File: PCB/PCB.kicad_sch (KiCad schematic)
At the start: 38 parts, among them J1 USB_B_Mini, J2 Conn_02x03_Odd_Even, J3 OLED, J4 AudioJack3, Q1 MMBF170, Q2 MMBF170, SW1 SW_Push, SW2 SW_Push, SW3 12CE3xxxxxxTx, SW4 SW_SPST, U1 ATtiny261A-M, U2 MCP73832-2-OT

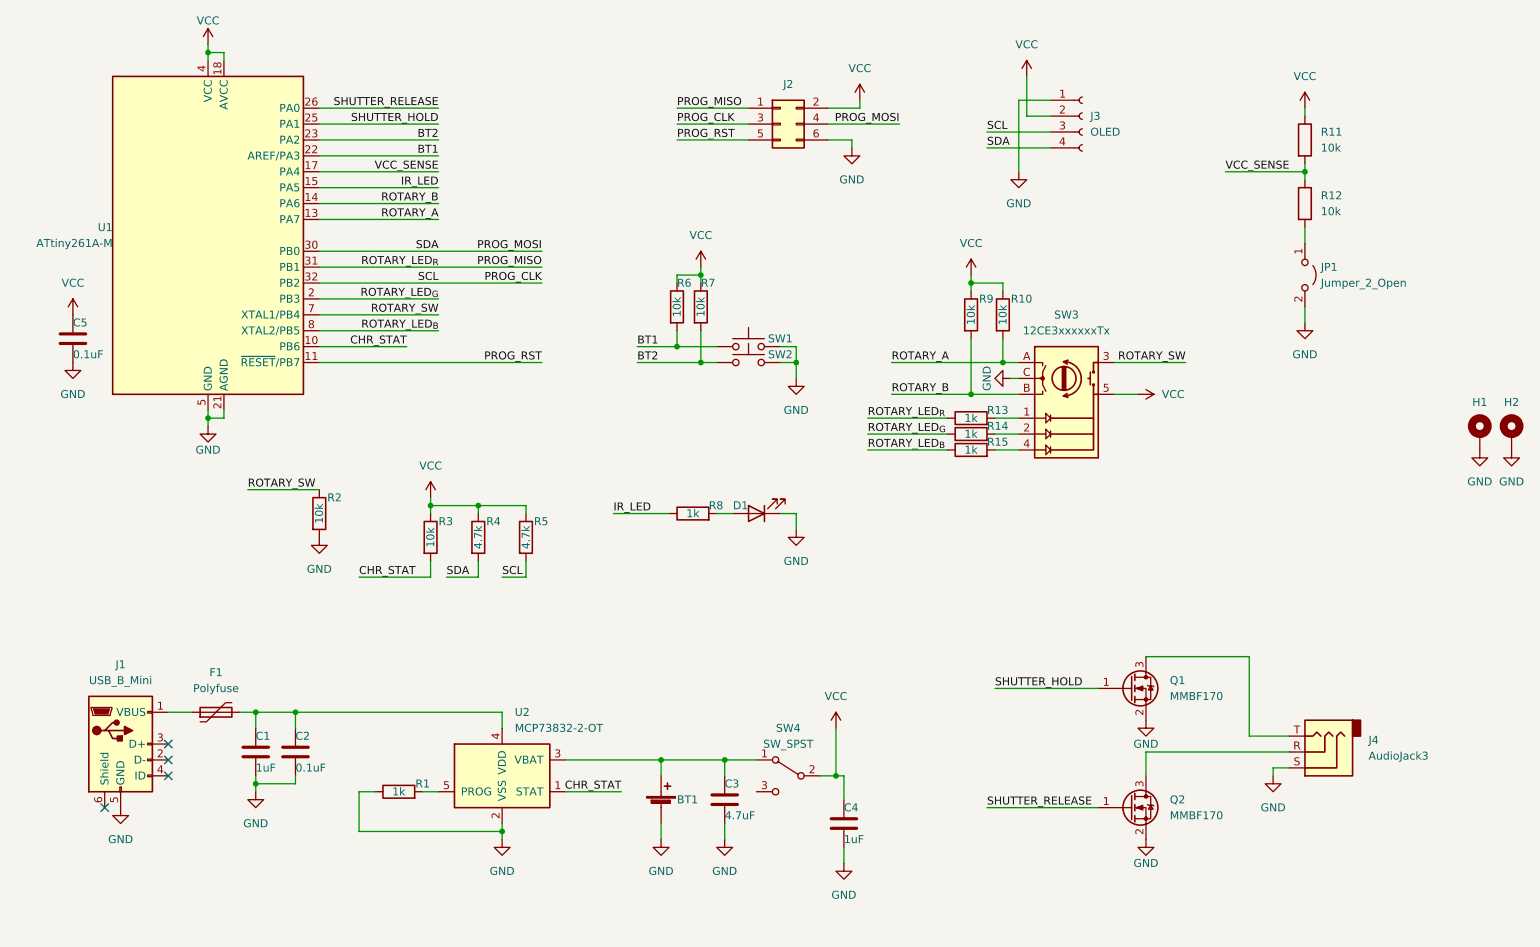
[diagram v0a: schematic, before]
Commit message: Updated schematic
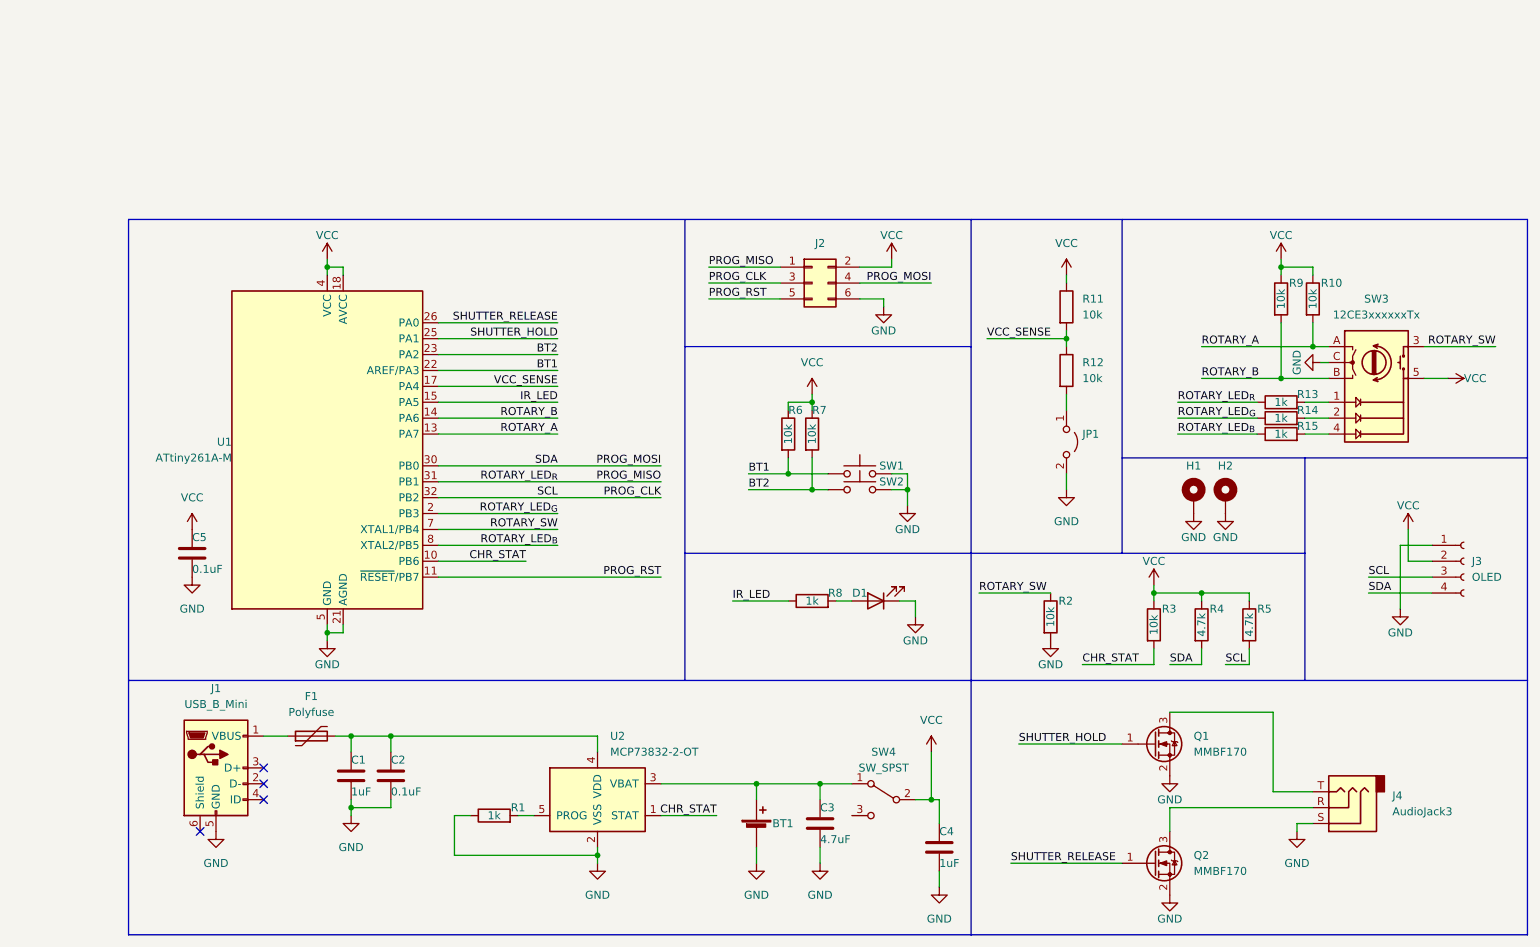
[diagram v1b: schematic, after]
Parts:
- JP1: value Jumper_2_Open -> (none); footprint Jumper:SolderJumper-2_P1.3mm_Open_RoundedPad1.0x1.5mm -> (none)
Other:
- title: (none) -> Remote Camera Shutter
- moved on the sheet: BT1, C1, C2, C3, C4, C5, D1, F1, H1, H2, J1, J2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
